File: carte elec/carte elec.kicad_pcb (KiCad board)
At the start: 2 copper layers, 135 x 115 mm, 51 parts, among them J1 SD_Card_Device, J2 Barrel_Jack_Switch, U1 ESP32-S3-UNO, U2 R-78E5.0-1.0

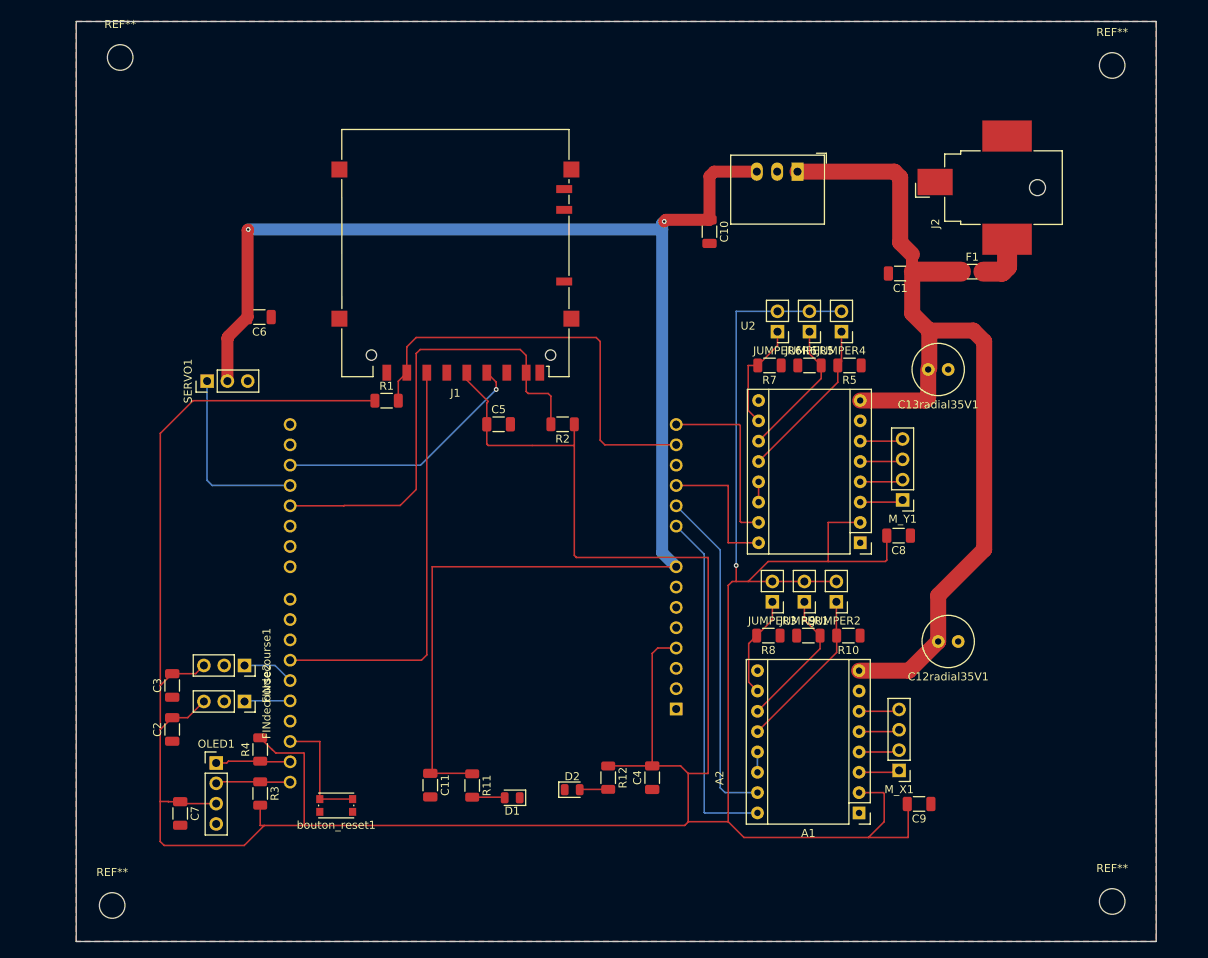
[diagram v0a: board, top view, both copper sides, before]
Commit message: Add files via upload
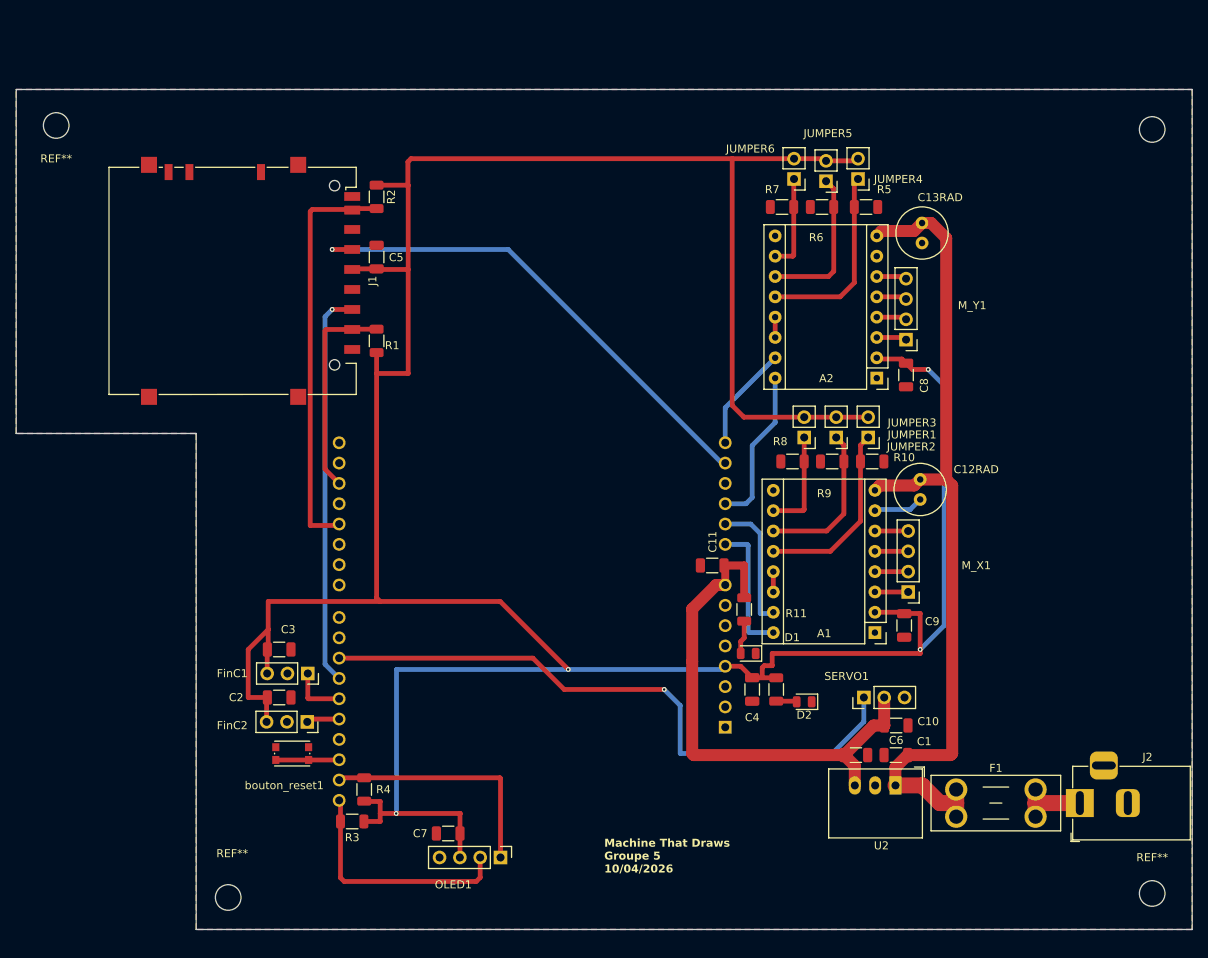
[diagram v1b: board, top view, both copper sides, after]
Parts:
- F1: footprint Fuse:Fuse_1206_3216Metric -> Fuse:Fuseholder_Blade_Mini_Keystone_3568
- J2: footprint Connector_BarrelJack:BarrelJack_CUI_PJ-036AH-SMT_Horizontal -> Connector_BarrelJack:BarrelJack_Horizontal
- moved REF** 166.0 mm to (209.0, 147.0), turned to 180 degrees
- moved REF** 163.8 mm to (72.0, 51.0), turned to 180 degrees
- moved REF** 162.2 mm to (209.0, 51.5), turned to 180 degrees
- moved REF** 151.7 mm to (93.5, 147.5), turned to 180 degrees
- moved C6 94.6 mm to (177.0, 126.0)
- moved SERVO1 91.1 mm to (173.0, 122.5)
- moved J2 77.9 mm to (200.0, 135.7), turned to 180 degrees
- moved U2 77.7 mm to (176.9, 133.5)
- moved C10 67.9 mm to (172.0, 129.7), turned to 0 degrees
- moved F1 64.8 mm to (184.5, 134.0)
- moved C1 60.2 mm to (177.0, 129.7)
- moved C11 44.7 mm to (154.0, 106.0), turned to 180 degrees
- moved R11 40.5 mm to (158.0, 111.5)
- moved OLED1 37.5 mm to (127.5, 142.5), turned to -90 degrees
- moved R2 36.7 mm to (112.0, 59.9), turned to -90 degrees
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- renumbered C12radial35V1 to C12RAD, C13radial35V1 to C13RAD, FINdecourse1 to FinC1, FINdecourse2 to FinC2
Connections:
- J2 pad 1: GND -> Net-(F1-Pad2)
- J2 pad 2: Net-(F1-Pad2) -> GND
- J2 pad 3: unconnected-(J2-Pad3) -> GND
- U1 pad 13: CS_SD -> SCK
- U1 pad 17: SCK -> CS_SD
- U1 pad 18: SERVO -> unconnected-(U1-GPIO17/ADC2_CH6-Pad18)
- U1 pad 25: unconnected-(U1-GPIO10/ADC1_CH9-Pad25) -> SERVO
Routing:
- net +5V: track 194.8 -> 66.0 mm, vias 2 -> 0
- net +3V3: track 466.1 -> 408.7 mm, vias 1 -> 4
- net SERVO: track 23.1 -> 78.7 mm, vias 0 -> 1
- net SCK: track 32.3 -> 62.7 mm
- net CS_SD: track 54.1 -> 26.4 mm
- net DIR_X: track 43.9 -> 16.9 mm
- net STEP_X: track 42.4 -> 17.1 mm
- net SDA: track 9.37 -> 30.2 mm
- net SDL: track 9.34 -> 30.1 mm
- net +12V: track 115.8 -> 106.3 mm
- net STEP_Y: track 22.4 -> 13.2 mm
- net MISO: track 59.2 -> 51.5 mm
- net BOUT: track 15.0 -> 7.93 mm
- net GND: track 0.00 -> 6.24 mm
- net Net-(A2-MS3): track 20.5 -> 23.8 mm
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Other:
- board size 135 x 115 mm -> 147 x 105 mm
- board text added: "Machine That Draws Groupe 5 10/04/2026"
